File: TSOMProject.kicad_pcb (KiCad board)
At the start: 2 copper layers, 64 parts, among them IC1 TCAN337DCNR, IC2 TCAN337DCNR, J10 Conn_02x02_Odd_Even, J11 GPS_I2C, J12 GPS_BAT, J14 Barrel_Jack_Switch, J3 Conn_Coaxial, J4 Conn_02x06_Counter_Clockwise, J5 Conn_02x07_Vertical, J6 To The Zedboard, J8 Conn_02x06_Odd_Even, J9 Conn_02x05_Counter_Clockwise, SW4 GPS_RESET, U1 ASM330LHHTR, U10 TPS54560BDDA, U7 CDSOT23-T24CAN, U8 CDSOT23-T24CAN, U9 PA1616S_GPS

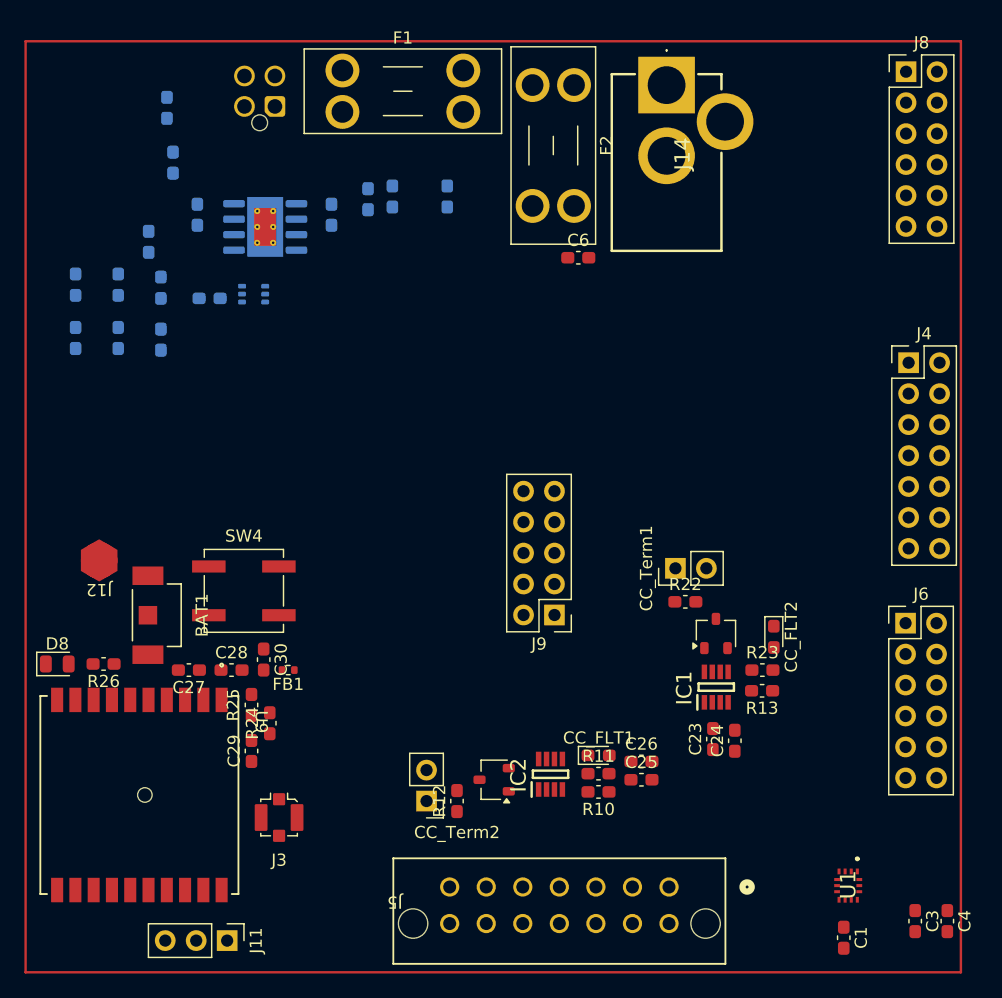
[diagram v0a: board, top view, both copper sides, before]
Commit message: more layout
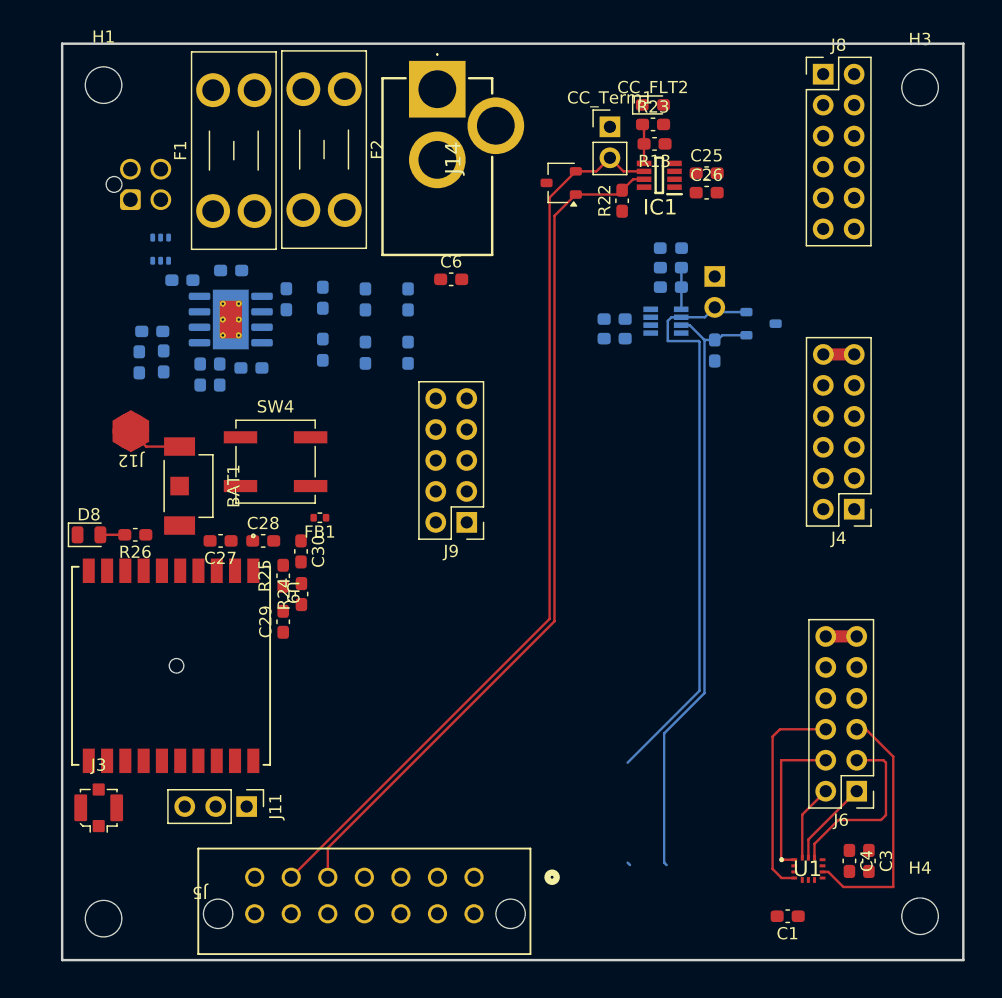
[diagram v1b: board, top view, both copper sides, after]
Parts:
- added H1: M.3, MountingHole:MountingHole_3mm, F.Cu at (138.4, 89.4)
- added H2: M.3, MountingHole:MountingHole_3mm, F.Cu at (138.4, 157.8)
- added H3: M.3, MountingHole:MountingHole_3mm, F.Cu at (205.4, 89.6)
- added H4: M.3, MountingHole:MountingHole_3mm, F.Cu at (205.4, 157.6)
- C23, C24, CC_FLT1, CC_Term2, IC2, R10, R11, R12, U7: moved to B.Cu
- J4: footprint Connector_PinHeader_2.54mm:PinHeader_2x07_P2.54mm_Vertical -> Connector_PinHeader_2.54mm:PinHeader_2x06_P2.54mm_Vertical
- moved C25 50.1 mm to (187.9, 96.6)
- moved CC_Term2 49.1 mm to (188.6, 105.1)
- moved C26 47.0 mm to (187.9, 98.2)
- moved R13 45.7 mm to (183.6, 94.2)
- moved R23 45.7 mm to (183.5, 92.6)
- moved CC_FLT2 44.8 mm to (183.5, 91.0), turned to 0 degrees
- moved U7 43.4 mm to (192.3, 109.0), turned to 0 degrees
- moved R12 42.6 mm to (188.6, 111.2)
- moved IC1 42.3 mm to (184.0, 96.8), turned to 180 degrees
- moved CC_FLT1 42.0 mm to (184.9, 102.8), turned to 180 degrees
- moved R11 41.9 mm to (184.9, 104.4), turned to 180 degrees
- moved R10 41.8 mm to (184.9, 106.0), turned to 0 degrees
- moved U8 39.1 mm to (175.9, 97.4), turned to 180 degrees
- moved IC2 38.4 mm to (184.6, 108.8), turned to 0 degrees
- moved CC_Term1 36.6 mm to (179.9, 92.8), turned to 0 degrees
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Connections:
- C4 pad 1: +3.3V -> unconnected-(C4-Pad1)
- C4 pad 2: GND -> unconnected-(C4-Pad2)
- CC_Term1 pad 2: TelCAN_L -> TelCAN_L-
- CC_Term2 pad 2: CarCAN_L -> CarCAN_L-
- IC1 pad 6: TelCAN_L -> TelCAN_L-
- IC1 pad 7: TelCAN_H -> TelCAN_H+
- IC2 pad 6: CarCAN_L -> CarCAN_L-
- IC2 pad 7: CarCAN_H -> CarCAN_H+
- J4 pad 1: IMU_MOSI -> /Connector/TP1
- J4 pad 2: IMU_CS -> /Connector/TP4
- J4 pad 5: GPS_SCL -> GPS_SDA
- J4 pad 6: IMU_MISO -> /Connector/TP2
- J4 pad 7: GPS_SDA -> GPS_SCL
- J4 pad 8: IMU_CLK -> /Connector/TP5
- J5 pad 10: CarCAN_TX -> CarCAN_L-
- J5 pad 12: TelCAN_TX -> TelCAN_H+
- J5 pad 13: TelCAN_TX -> TelCAN_L-
- J5 pad 2: CarCAN_H -> CarCAN_H+
- J5 pad 3: CarCAN_RX -> CarCAN_L-
- J5 pad 5: TelCAN_RX -> TelCAN_H+
- J5 pad 6: TelCAN_RX -> TelCAN_L-
- J5 pad 9: CarCAN_TX -> CarCAN_H+
- J6 pad 1: IMU_INT1 -> IMU_CLK
- J6 pad 2: IMU_INT2 -> IMU_MOSI
- J6 pad 3: /Connector/TP1 -> IMU_CS
- J6 pad 4: /Connector/TP4 -> IMU_MISO
- J6 pad 5: /Connector/TP2 -> IMU_INT2
- J6 pad 6: /Connector/TP5 -> IMU_INT1
- J6 pad 7: /Connector/TP3 -> unconnected-(J6-Pin_7-Pad7)
- J6 pad 8: /Connector/TP6 -> unconnected-(J6-Pin_8-Pad8)
- J8 pad 11: CarCAN_RX -> TelCAN_TX
- J8 pad 5: CarCAN_TX -> TelCAN_RX
- J8 pad 7: TelCAN_TX -> CarCAN_RX
- J8 pad 9: TelCAN_RX -> CarCAN_TX
- J9 pad 10: /Connector/TP4 -> /Connector/TP2
- J9 pad 2: /Connector/TP2 -> /Connector/TP4
- R11 pad 1: unconnected-(R11-Pad1) -> /CAN/CarCAN_Fault
- R12 pad 2: CarCAN_H -> CarCAN_H+
- R22 pad 2: TelCAN_H -> TelCAN_H+
- U7 pad 1: CarCAN_H -> CarCAN_H+
- U7 pad 2: CarCAN_L -> CarCAN_L-
- U8 pad 1: TelCAN_H -> TelCAN_H+
- U8 pad 2: TelCAN_L -> TelCAN_L-
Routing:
- net TelCAN_L-: track 0.00 -> 74.1 mm
- net TelCAN_H+: track 0.00 -> 70.6 mm
- net CarCAN_H+: track 0.00 -> 50.6 mm
- net CarCAN_L-: track 0.00 -> 48.6 mm
- net IMU_INT2: track 0.00 -> 20.9 mm
- net IMU_INT1: track 0.00 -> 17.6 mm
- net IMU_CS: track 0.00 -> 14.8 mm
- net IMU_MISO: track 0.00 -> 12.9 mm
- net IMU_CLK: track 0.00 -> 7.10 mm
- net IMU_MOSI: track 0.00 -> 6.26 mm
- net +3V3: track 0.00 -> 5.08 mm
- net /GPS/+3.3V_GPS_BAT: track 0.00 -> 4.52 mm
- net /CAN/CarCAN_Fault: track 0.00 -> 3.43 mm
- net /CAN/TelCAN_Fault: track 0.00 -> 3.25 mm
- net /GPS/GPS_D8: track 0.00 -> 2.00 mm
- added copper zone on B.Cu, net GND
- added copper zone on F.Cu, net GND
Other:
- board outline added: 73.9 x 75.2 mm
- board text added: "21.59 mm (0.850 in)"
- board text added: "44.20 mm (1.748 in)"
- board text added: "67.41 mm (2.654 in)"
